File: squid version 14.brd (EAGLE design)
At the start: 33 x 61 mm, 62 parts, among them J2 ATMEL_PROGRAMMER_HEADERNL, U2 MCP73832

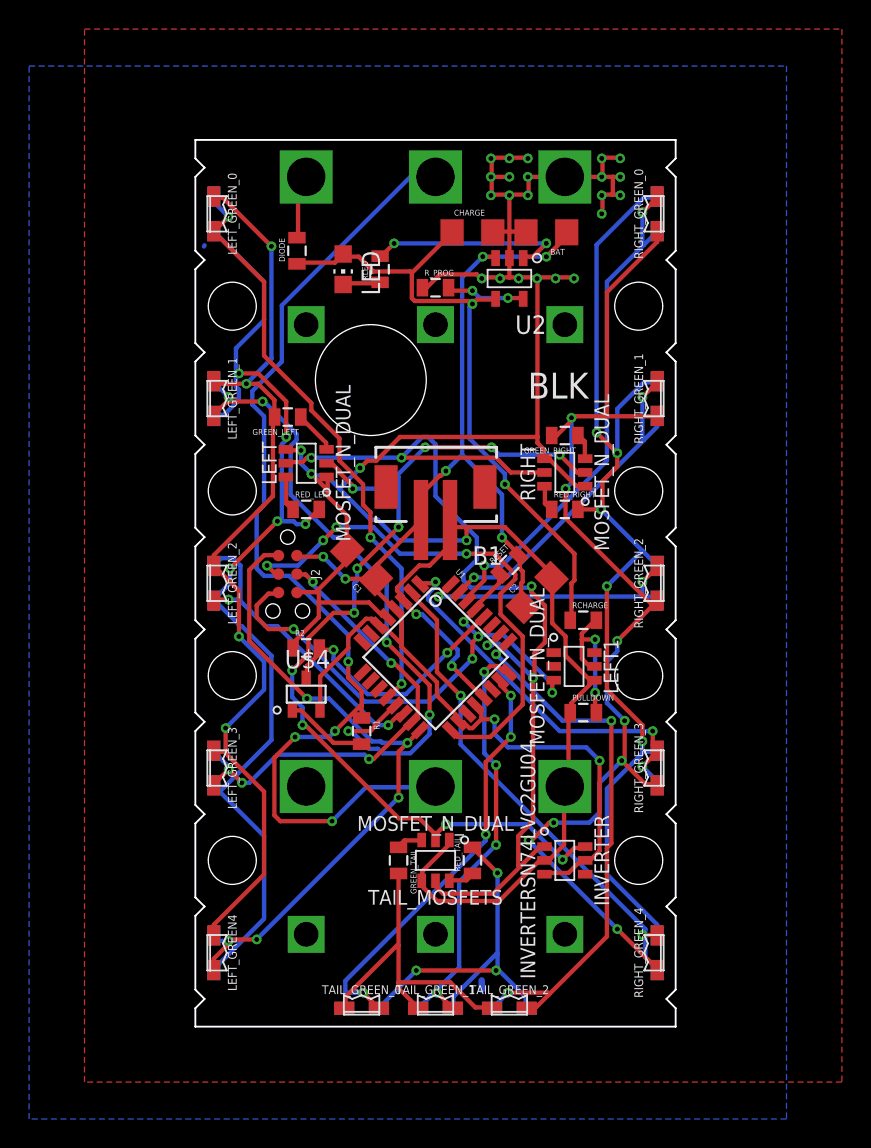
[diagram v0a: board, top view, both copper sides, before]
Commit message: small test change
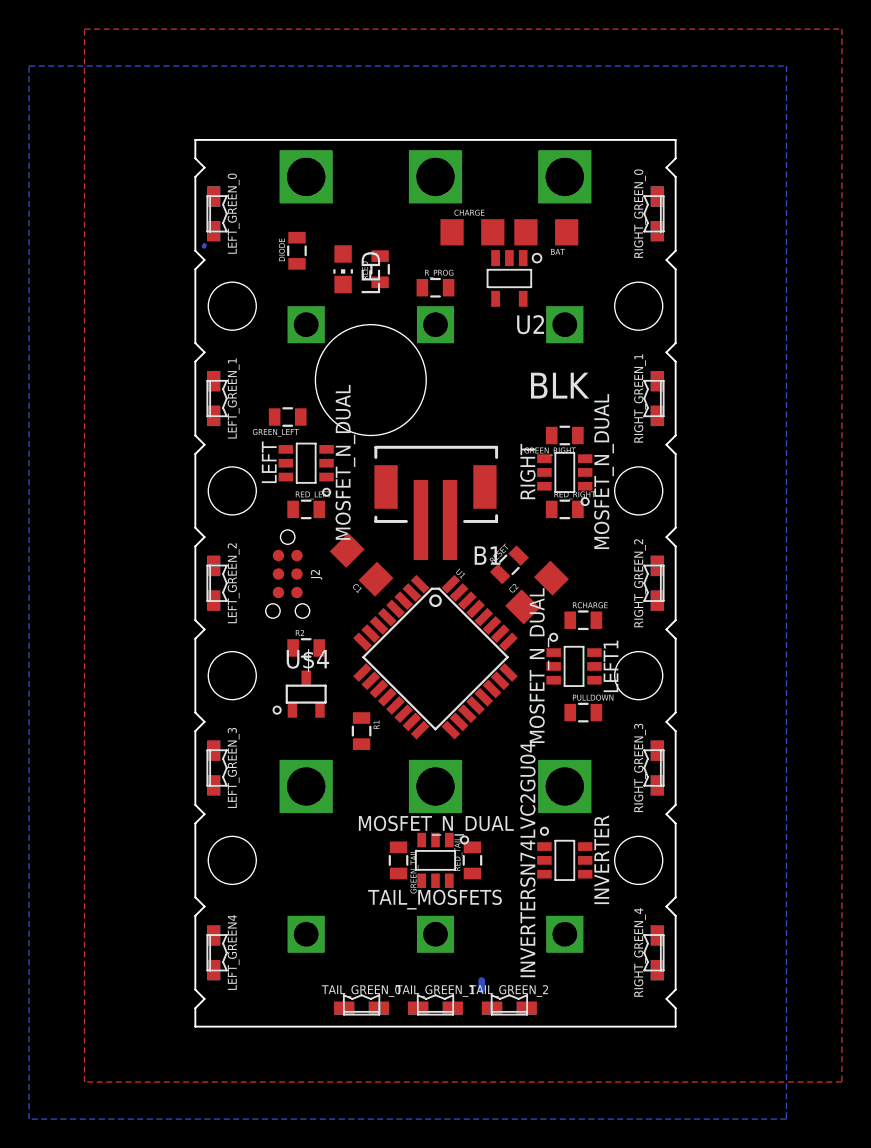
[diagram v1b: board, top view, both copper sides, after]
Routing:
- net GND: track 175.3 -> 0.00 mm, vias 28 -> 0
- net VBAT: track 99.7 -> 0.00 mm, vias 8 -> 0
- net N$11: track 76.8 -> 0.00 mm, vias 8 -> 0
- net N$7: track 72.6 -> 0.00 mm, vias 5 -> 0
- net N$9: track 71.7 -> 0.00 mm, vias 4 -> 0
- net RED_LEFT_CATHODE: track 71.6 -> 0.00 mm, vias 5 -> 0
- net N$12: track 70.5 -> 0.00 mm, vias 5 -> 0
- net N$2: track 66.9 -> 0.00 mm, vias 11 -> 0
- net GREEN_LEFT_CATHODE: track 64.8 -> 0.00 mm, vias 4 -> 0
- net PB4: track 45.7 -> 0.00 mm, vias 5 -> 0
- net N$21: track 45.6 -> 0.00 mm, vias 2 -> 0
- net PB1: track 44.7 -> 0.00 mm, vias 5 -> 0
- net PB0: track 41.1 -> 0.00 mm, vias 3 -> 0
- net PC2: track 38.0 -> 0.00 mm, vias 3 -> 0
- net RESET: track 36.7 -> 0.00 mm, vias 5 -> 0
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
